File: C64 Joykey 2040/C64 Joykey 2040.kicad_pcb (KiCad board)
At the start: 2 copper layers, 99.7 x 74.9 mm, 69 parts, among them J1 Port_1, J2 Port_2, J4 Expansion, M1 Mounting, M2 Mounting, M3 Mounting, M4 Mounting, Q1 2N3904, SW1 UP, SW10 P1_FIRE2, SW11 P2_FIRE3, SW12 P1_FIRE5, SW13 P1_FIRE6, SW2 DOWN, SW3 LEFT, SW4 RIGHT, SW5 P1_FIRE4, SW6 P2_FIRE1, SW7 P1_FIRE1, SW8 P1_FIRE3, SW9 P2_FIRE2, U1 RP2040-Zero

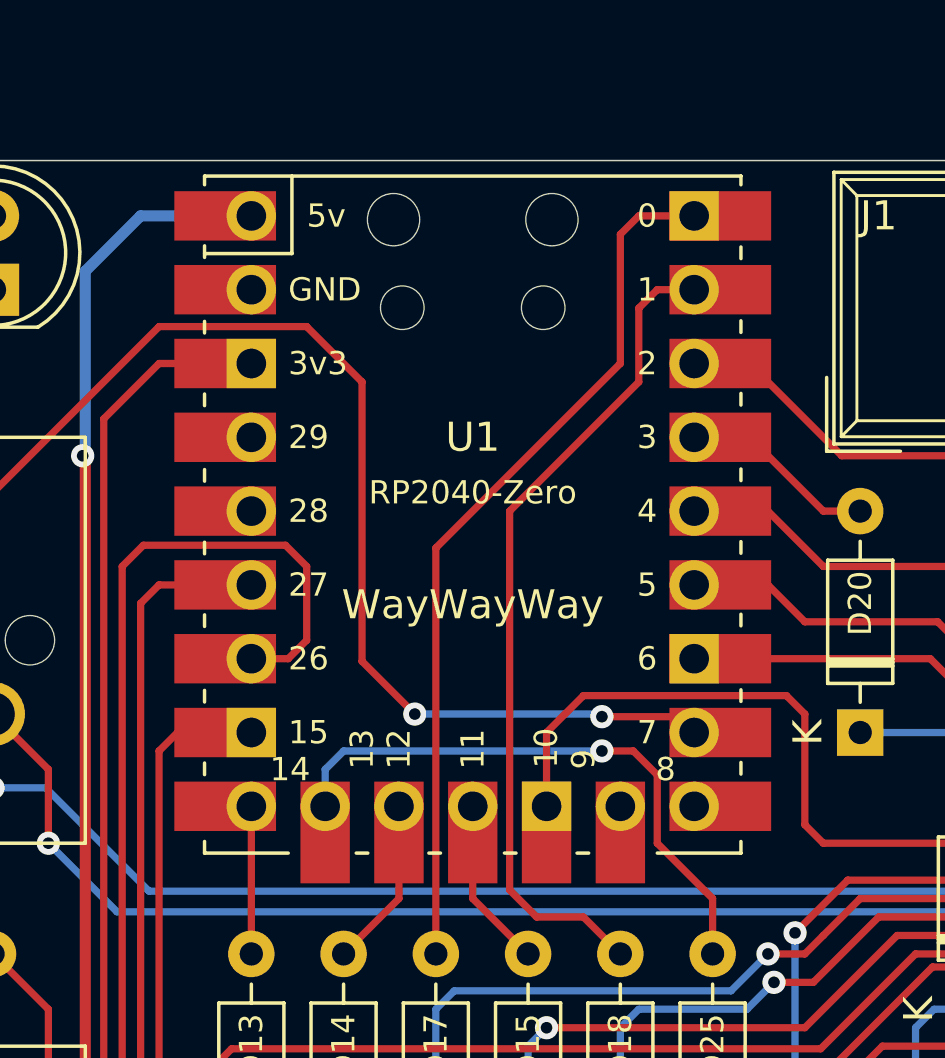
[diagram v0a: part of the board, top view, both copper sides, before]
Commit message: Slight build tweaks for clarity
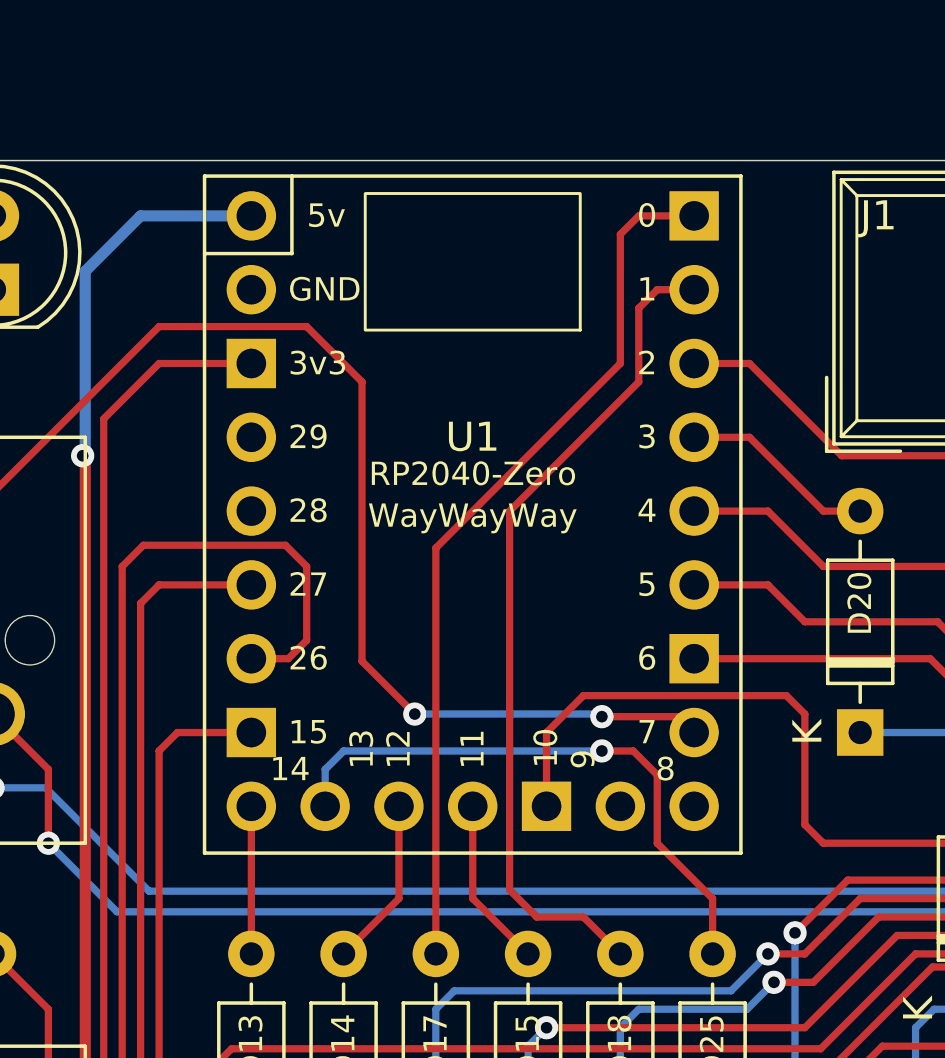
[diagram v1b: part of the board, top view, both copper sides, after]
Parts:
- U1: footprint pi_pico:RP2040-Zero -> pi_pico:RP2040-Zero-THT
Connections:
- net /L2_1 renamed /L2
- net /R2_1 renamed /R2
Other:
- board text added: "Always configure FIRE2/FIRE3 polarity according to what's required by the system. Leave unjumpered (N/C) if you are not sure."
- board text added: "IMPORTANT!"
- board text added: "You break it, you fix it!"
- board text removed: "IMPORTANT! Always configure FIRE2/FIRE3 polarity according to what's required by the system. Leave unjumpered (N/C) if you are not sure. You break it, you fix it!"
